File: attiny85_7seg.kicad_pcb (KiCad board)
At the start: 2 copper layers, 55 x 61 mm, 26 parts, among them J1 Conn_01x06_Pin, J2 Conn_01x03_Pin, SW1 SW_Push, U1 ATtiny85, U2 CC56-12SURKWA, U3 74HC595, U4 74HC595

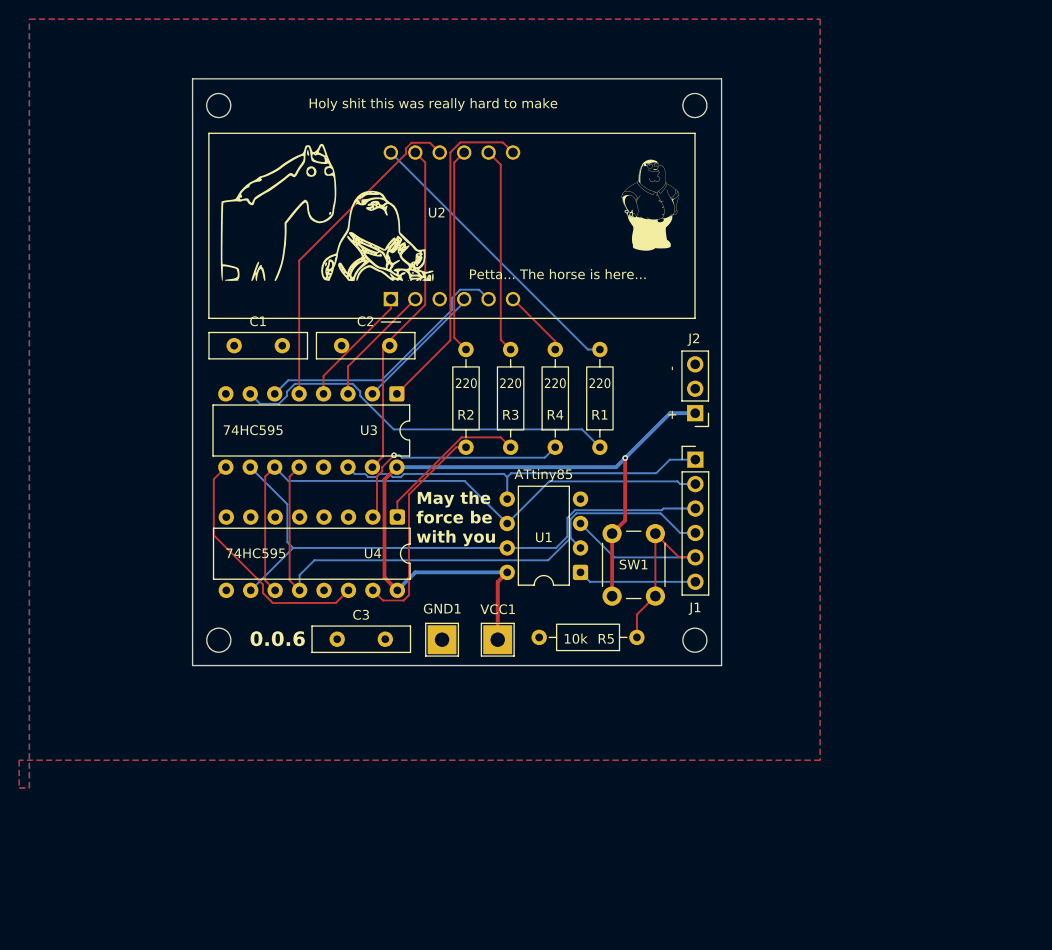
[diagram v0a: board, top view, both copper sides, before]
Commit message: v0.1.0
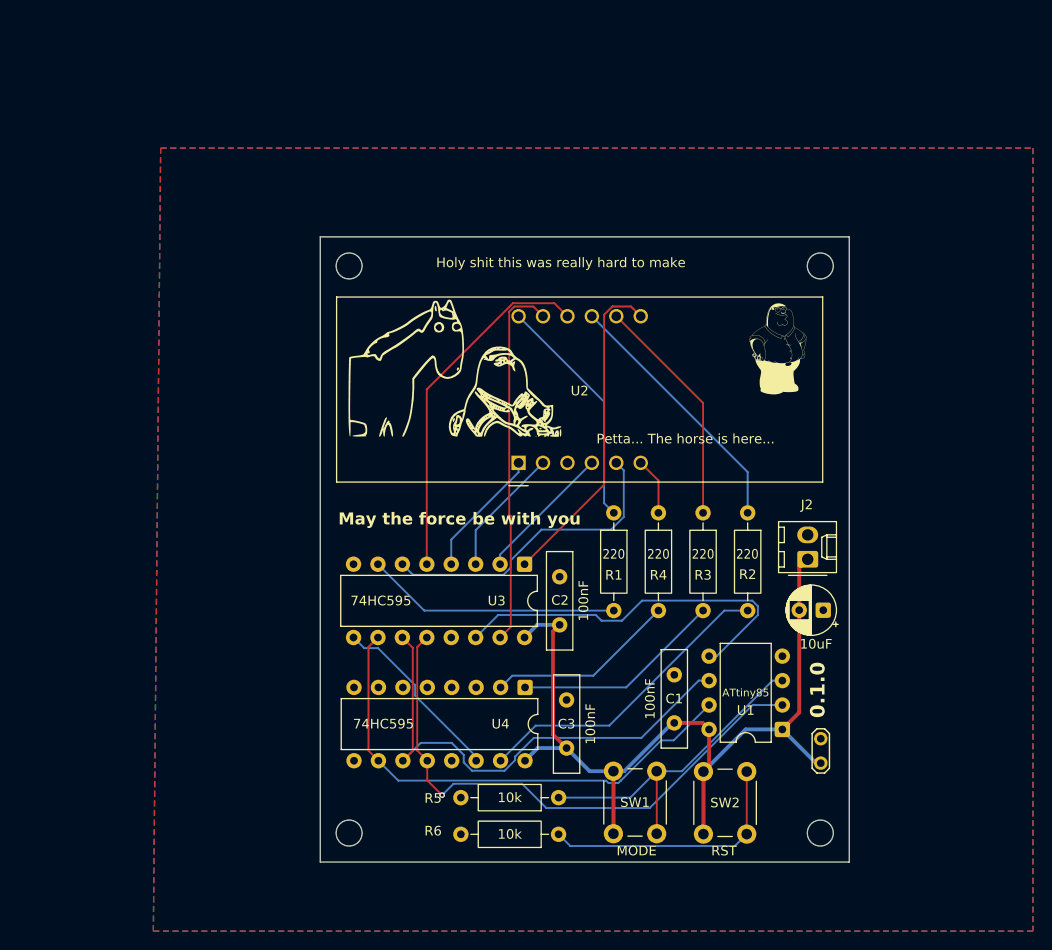
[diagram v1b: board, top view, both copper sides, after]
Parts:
- removed GND1, VCC1: TestPoint, TestPoint:TestPoint_THTPad_3.0x3.0mm_Drill1.5mm
- removed HOLE1, HOLE2, HOLE3, HOLE4: MountingHole_2.5mm, MountingHole:MountingHole_2.5mm
- removed IMG5: LOGO, SilkScreen:simbols
- removed J1: Conn_01x06_Pin, Connector_PinHeader_2.54mm:PinHeader_1x06_P2.54mm_Vertical
- added C4: 10uF, Capacitor_THT:CP_Radial_D5.0mm_P2.50mm, F.Cu at (170.7, 105.9)
- added H1: MountingHole, MountingHole:MountingHole_2.7mm_M2.5, F.Cu at (121.4, 129.1)
- added H2: MountingHole, MountingHole:MountingHole_2.7mm_M2.5, F.Cu at (170.4, 129.1)
- added H3: MountingHole, MountingHole:MountingHole_2.7mm_M2.5, F.Cu at (170.4, 70.1)
- added H4: MountingHole, MountingHole:MountingHole_2.7mm_M2.5, F.Cu at (121.4, 70.1)
- added R6: 10k, Resistor_THT:R_Axial_DIN0207_L6.3mm_D2.5mm_P10.16mm_Horizontal, F.Cu at (143.2, 129.2)
- added SW2: SW_Push, Button_Switch_THT:SW_PUSH_6mm, F.Cu at (162.7, 122.7)
- added TP1: TestPoint_2Pole, TestPoint:TestPoint_2Pads_Pitch2.54mm_Drill0.8mm, F.Cu at (170.4, 121.8)
- C1, C2, C3: value 10uF -> 100nF
- J2: value Conn_01x03_Pin -> Conn_01x02_Pin; footprint Connector_PinHeader_2.54mm:PinHeader_1x03_P2.54mm_Vertical -> Connector_Molex:Molex_KK-254_AE-6410-02A_1x02_P2.54mm_Vertical
- moved C1 57.1 mm to (155.2, 112.6), turned to -90 degrees
- moved C2 36.8 mm to (143.3, 107.4), turned to 90 degrees
- moved R2 30.1 mm to (162.8, 95.8), turned to -90 degrees
- moved U1 26.6 mm to (166.4, 118.3)
- moved C3 26.4 mm to (144.0, 120.3), turned to 90 degrees
- moved SW1 24.7 mm to (153.4, 122.7)
- moved IMG2 22.7 mm to (123.4, 85.5)
- moved U4 22.1 mm to (139.7, 114.0)
- moved U3 22.1 mm to (139.6, 101.1)
- moved IMG3 21.9 mm to (167.5, 85.5)
- moved U2 21.6 mm to (139.0, 90.6)
- moved R3 21.1 mm to (158.2, 95.8), turned to -90 degrees
- moved LOGO1 20.9 mm to (130.3, 77.8)
- moved IMG1 20.0 mm to (165.9, 78.7)
- moved J2 19.2 mm to (169.1, 100.6), turned to 90 degrees
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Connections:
- net /PB0 renamed /DATA
- net /PB1 renamed /SRCLK
- net /PB2 renamed /SRCLR
- net /PB3 renamed /RCLK
- net /PB4 renamed /MODE
- net Net-(U2-a) renamed /QA
- net Net-(U2-b) renamed /QB
- net Net-(U2-c) renamed /QC
- net Net-(U2-d) renamed /QD
- net Net-(U2-e) renamed /QE
- net Net-(U2-f) renamed /QF
- net Net-(U2-g) renamed /QG
- C1 pad 1: VCC -> GND
- C1 pad 2: GND -> VCC
- J2 pad 2: unconnected-(J2-Pin_2-Pad2) -> GND
- R1 pad 1: Net-(U3-QH) -> Net-(U2-CC1)
- R1 pad 2: Net-(U2-CC1) -> /D1
- R2 pad 1: Net-(U4-QA) -> Net-(U2-CC2)
- R2 pad 2: Net-(U2-CC2) -> /D2
- R3 pad 1: Net-(U4-QB) -> Net-(U2-CC3)
- R3 pad 2: Net-(U2-CC3) -> /D3
- R4 pad 1: Net-(U4-QC) -> Net-(U2-CC4)
- R4 pad 2: Net-(U2-CC4) -> /D4
- U1 pad 1: /PB5 -> VCC
- U3 pad 7: Net-(U3-QH) -> /D1
- U4 pad 1: Net-(U4-QB) -> /D3
- U4 pad 15: Net-(U4-QA) -> /D2
- U4 pad 2: Net-(U4-QC) -> /D4
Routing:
- net Net-(U3-QH): track 40.9 -> 0.00 mm
- net /D2: track 0.00 -> 32.2 mm
- net Net-(R6-Pad1): track 0.00 -> 27.1 mm
- net /D1: track 0.00 -> 26.5 mm
- net Net-(U4-QC): track 24.6 -> 0.00 mm, vias 1 -> 0
- net Net-(U4-QA): track 22.8 -> 0.00 mm
- net /D3: track 0.00 -> 21.8 mm
- net /D4: track 0.00 -> 19.7 mm
- net Net-(U4-QB): track 16.6 -> 0.00 mm
- net /PB5: track 12.4 -> 0.00 mm
- net VCC: track 81.8 -> 92.8 mm, vias 1 -> 0
- net /SRCLK: track 61.8 -> 52.0 mm
- net /SRCLR: track 61.1 -> 52.3 mm
- net Net-(U3-QH'): track 25.6 -> 18.9 mm
- net Net-(U2-CC2): track 21.4 -> 27.2 mm
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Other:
- board size 55 x 61 mm -> 55 x 65 mm
- board text added: "MODE"
- board text added: "Pin headers used only for programming Attiny85"
- board text added: "RST"
- board text removed: "+"
- board text removed: "-"
